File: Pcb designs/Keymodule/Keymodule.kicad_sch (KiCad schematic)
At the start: 105 parts, among them J1 USB connect, U1 RP2040, U2 SN74LV1T34DBV, U3 AMS1117-3.3, U4 W25Q128JVS, Y1 ABM8-272-T3

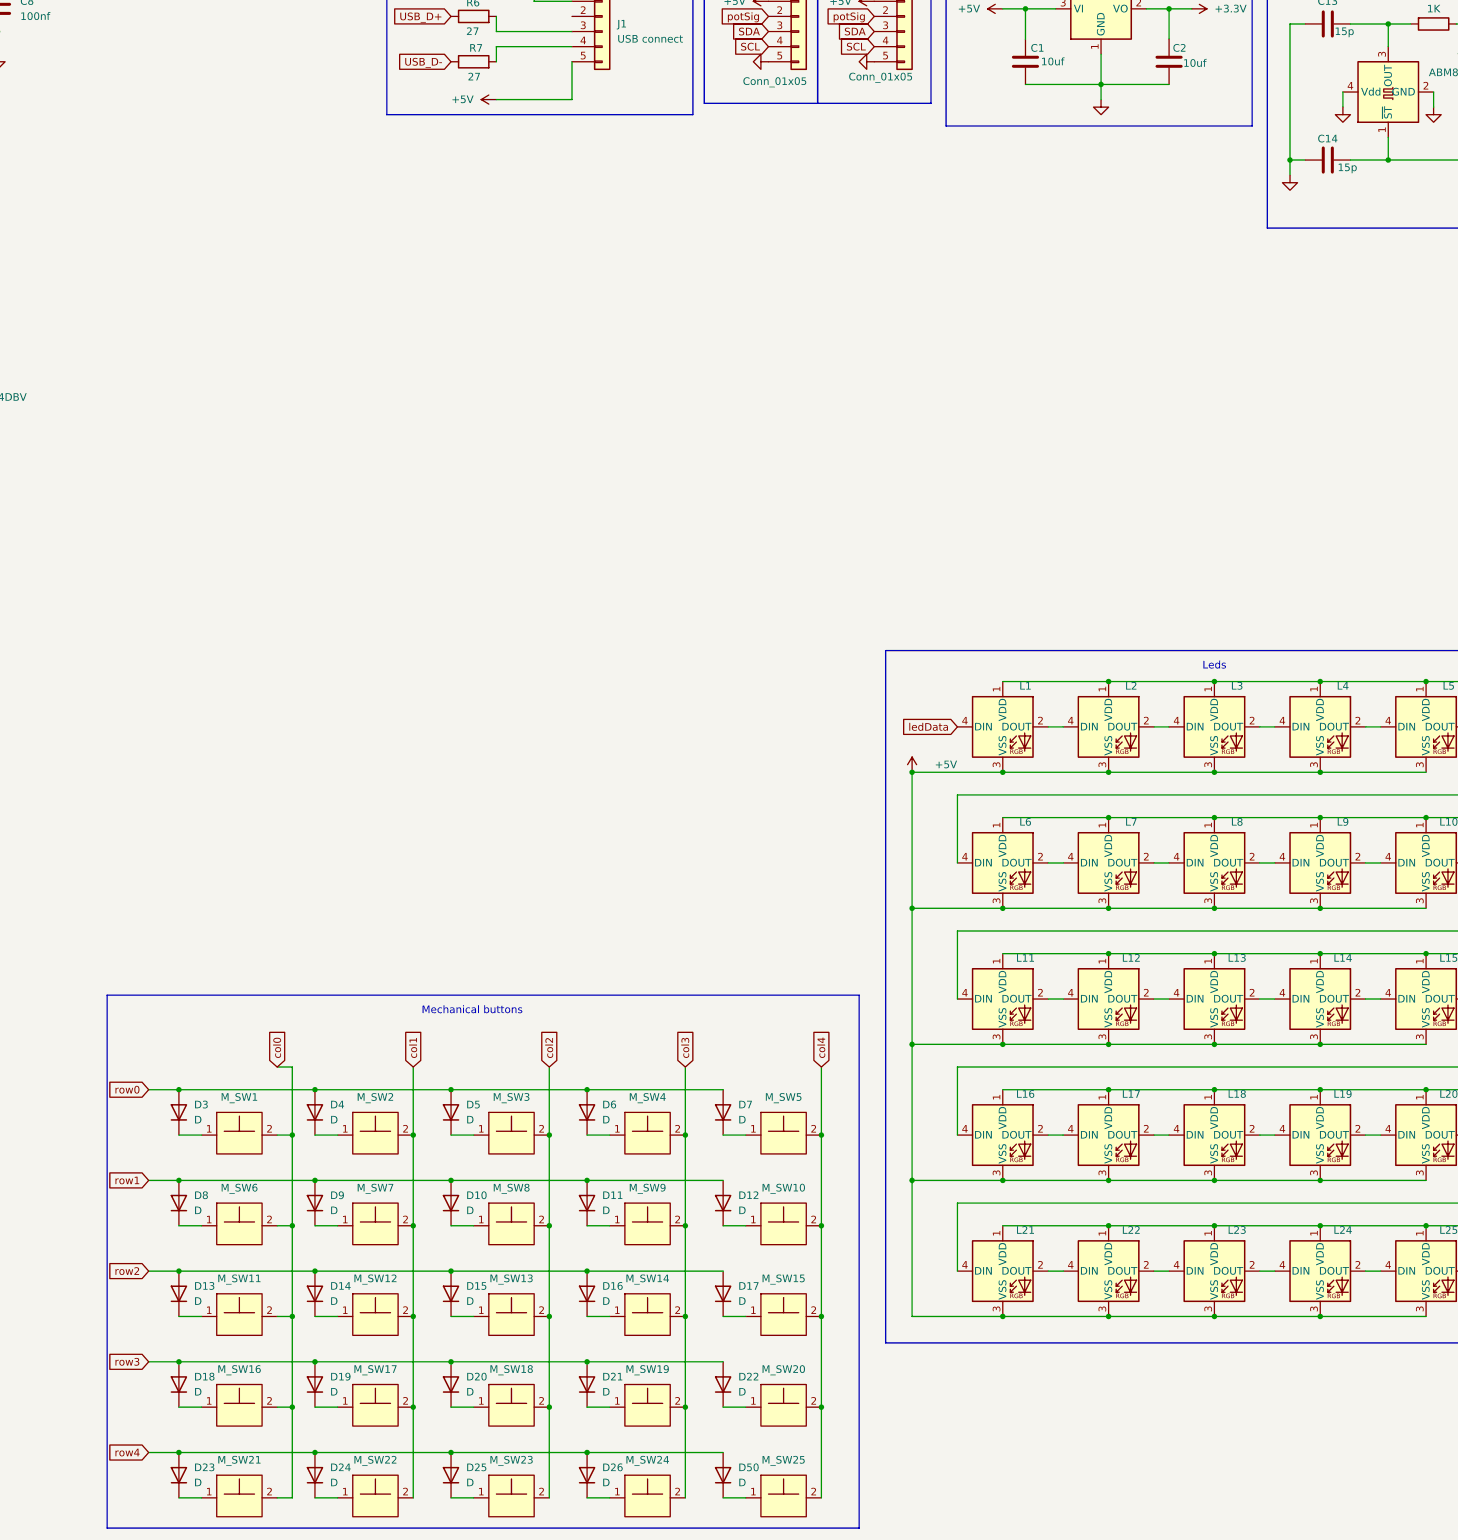
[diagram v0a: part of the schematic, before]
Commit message: Stared wiring ic
LED signal boost not done
But its a start
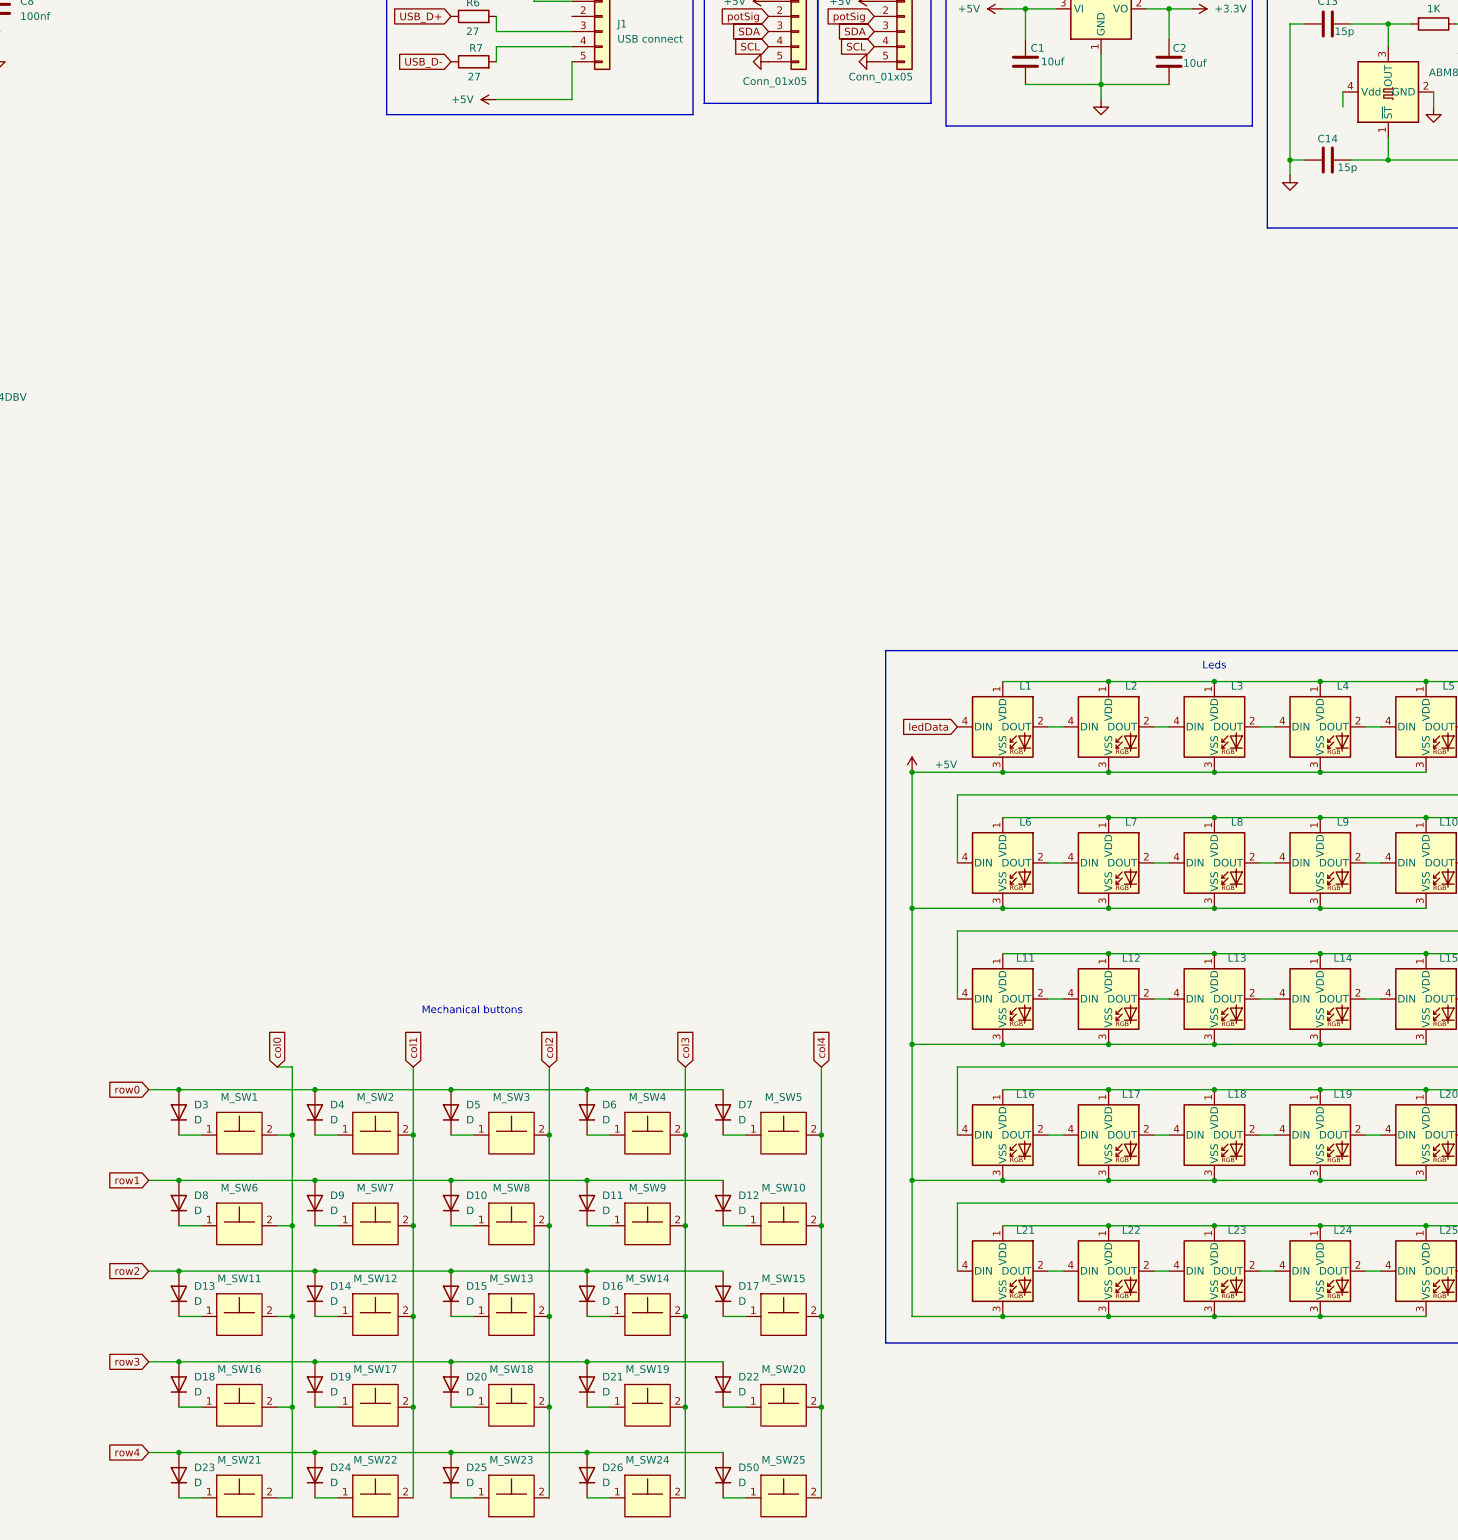
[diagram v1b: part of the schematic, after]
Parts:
- M_SW1, M_SW10, M_SW11, M_SW12, M_SW13, M_SW14, M_SW15, M_SW16, M_SW17, M_SW18, M_SW19, M_SW2, M_SW20, M_SW21, M_SW22, M_SW23, M_SW24, M_SW25, M_SW3, M_SW4, M_SW5, M_SW6, M_SW7, M_SW8, M_SW9: footprint 1_Custom_library:Kailh Switch 1350 -> 1_Custom_library:Kailh low profile Choc switch V1
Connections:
- net GND: no longer Y1.4 (Vdd)
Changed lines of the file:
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@@
 	)
 	(rectangle
-		(start 167.005 191.135)
-		(end 293.37 280.67)
-		(stroke
-			(width 0)
-			(type solid)
-		)
-		(fill
-			(type color)
-			(color 120 120 120 0.38)
-		)
-	)
-	(rectangle
 		(start 213.995 14.605)
 		(end 265.43 43.18)
@@
 			)
 		)
-		(property "Footprint" "1_Custom_library:Kailh Switch 1350"
+		(property "Footprint" "1_Custom_library:Kailh low profile Choc switch V1"
 			(at 280.67 231.14 0)
 			(effects
@@
 			)
 		)
-		(property "Footprint" "1_Custom_library:Kailh Switch 1350"
+		(property "Footprint" "1_Custom_library:Kailh low profile Choc switch V1"
 			(at 212.09 276.86 0)
 			(effects
@@
 			)
 		)
-		(property "Footprint" "1_Custom_library:Kailh Switch 1350"
+		(property "Footprint" "1_Custom_library:Kailh low profile Choc switch V1"
 			(at 234.95 231.14 0)
 			(effects
@@
 			)
 		)
-		(property "Footprint" "1_Custom_library:Kailh Switch 1350"
+		(property "Footprint" "1_Custom_library:Kailh low profile Choc switch V1"
 			(at 189.23 276.86 0)
 			(effects
@@
 			)
 		)
-		(property "Footprint" "1_Custom_library:Kailh Switch 1350"
+		(property "Footprint" "1_Custom_library:Kailh low profile Choc switch V1"
 			(at 234.95 276.86 0)
 			(effects
@@
 			)
 		)
-		(property "Footprint" "1_Custom_library:Kailh Switch 1350"
+		(property "Footprint" "1_Custom_library:Kailh low profile Choc switch V1"
 			(at 212.09 215.9 0)
 			(effects
@@
 			)
 		)
-		(property "Footprint" "1_Custom_library:Kailh Switch 1350"
+		(property "Footprint" "1_Custom_library:Kailh low profile Choc switch V1"
 			(at 189.23 246.38 0)
 			(effects
@@
 			)
 		)
-		(property "Footprint" "1_Custom_library:Kailh Switch 1350"
+		(property "Footprint" "1_Custom_library:Kailh low profile Choc switch V1"
 			(at 257.81 261.62 0)
 			(effects
@@
 			)
 		)
-		(property "Footprint" "1_Custom_library:Kailh Switch 1350"
+		(property "Footprint" "1_Custom_library:Kailh low profile Choc switch V1"
 			(at 257.81 231.14 0)
 			(effects
@@
 			)
 		)
-		(property "Footprint" "1_Custom_library:Kailh Switch 1350"
+		(property "Footprint" "1_Custom_library:Kailh low profile Choc switch V1"
 			(at 280.67 276.86 0)
 			(effects
@@
 			)
 		)
-		(property "Footprint" "1_Custom_library:Kailh Switch 1350"
+		(property "Footprint" "1_Custom_library:Kailh low profile Choc switch V1"
 			(at 257.81 246.38 0)
 			(effects
@@
 			)
 		)
-		(property "Footprint" "1_Custom_library:Kailh Switch 1350"
+		(property "Footprint" "1_Custom_library:Kailh low profile Choc switch V1"
 			(at 257.81 215.9 0)
 			(effects
@@
 			)
 		)
-		(property "Footprint" "1_Custom_library:Kailh Switch 1350"
+		(property "Footprint" "1_Custom_library:Kailh low profile Choc switch V1"
 			(at 189.23 215.9 0)
 			(effects
@@
 			)
 		)
-		(property "Footprint" "1_Custom_library:Kailh Switch 1350"
+		(property "Footprint" "1_Custom_library:Kailh low profile Choc switch V1"
 			(at 189.23 261.62 0)
 			(effects
@@
 			)
 		)
-		(property "Footprint" "1_Custom_library:Kailh Switch 1350"
+		(property "Footprint" "1_Custom_library:Kailh low profile Choc switch V1"
 			(at 212.09 231.14 0)
 			(effects
@@
 			)
 		)
-		(property "Footprint" "1_Custom_library:Kailh Switch 1350"
+		(property "Footprint" "1_Custom_library:Kailh low profile Choc switch V1"
 			(at 257.81 276.86 0)
 			(effects
@@
 			)
 		)
-		(property "Footprint" "1_Custom_library:Kailh Switch 1350"
+		(property "Footprint" "1_Custom_library:Kailh low profile Choc switch V1"
 			(at 234.95 246.38 0)
 			(effects
@@
 			)
 		)
-		(property "Footprint" "1_Custom_library:Kailh Switch 1350"
+		(property "Footprint" "1_Custom_library:Kailh low profile Choc switch V1"
 			(at 234.95 261.62 0)
 			(effects
@@
 	)
 	(symbol
-		(lib_id "power:GND")
-		(at 374.65 41.91 0)
-		(unit 1)
-		(exclude_from_sim no)
-		(in_bom yes)
-		(on_board yes)
-		(dnp no)
-		(fields_autoplaced yes)
-		(property "Reference" "#PWR028"
-			(at 374.65 48.26 0)
-			(effects
-				(font
-					(size 1.27 1.27)
-				)
-				(hide yes)
-			)
-		)
-		(property "Value" "GND"
-			(at 374.65 46.99 0)
-			(effects
-				(font
-					(size 1.27 1.27)
-				)
-				(hide yes)
-			)
-		)
-		(property "Footprint" ""
-			(at 374.65 41.91 0)
-			(effects
-				(font
-					(size 1.27 1.27)
-				)
-				(hide yes)
-			)
-		)
-		(property "Datasheet" ""
-			(at 374.65 41.91 0)
-			(effects
-				(font
-					(size 1.27 1.27)
-				)
-				(hide yes)
-			)
-		)
-		(property "Description" "Power symbol creates a global label with name \"GND\" , ground"
-			(at 374.65 41.91 0)
-			(effects
-				(font
-					(size 1.27 1.27)
-				)
-				(hide yes)
-			)
-		)
-		(pin "1"
-		)
-		(instances
-			(project "Keymodule"
-				(path "/8c3d34a5-d640-4303-a3a8-a4a01dc90234"
-					(reference "#PWR028")
-					(unit 1)
-				)
-			)
-		)
-	)
-	(symbol
 		(lib_id "Device:D")
 		(at 201.93 210.82 90)
@@
 			)
 		)
-		(property "Footprint" "1_Custom_library:Kailh Switch 1350"
+		(property "Footprint" "1_Custom_library:Kailh low profile Choc switch V1"
 			(at 212.09 246.38 0)
 			(effects
@@
 			)
 		)
-		(property "Footprint" "1_Custom_library:Kailh Switch 1350"
+		(property "Footprint" "1_Custom_library:Kailh low profile Choc switch V1"
 			(at 280.67 261.62 0)
 			(effects
@@
 			)
 		)
-		(property "Footprint" "1_Custom_library:Kailh Switch 1350"
+		(property "Footprint" "1_Custom_library:Kailh low profile Choc switch V1"
 			(at 280.67 246.38 0)
 			(effects
@@
 			)
 		)
-		(property "Footprint" "1_Custom_library:Kailh Switch 1350"
+		(property "Footprint" "1_Custom_library:Kailh low profile Choc switch V1"
 			(at 280.67 215.9 0)
 			(effects
@@
 			)
 		)
-		(property "Footprint" "1_Custom_library:Kailh Switch 1350"
+		(property "Footprint" "1_Custom_library:Kailh low profile Choc switch V1"
 			(at 189.23 231.14 0)
 			(effects
@@
 			)
 		)
-		(property "Footprint" "1_Custom_library:Kailh Switch 1350"
+		(property "Footprint" "1_Custom_library:Kailh low profile Choc switch V1"
 			(at 212.09 261.62 0)
 			(effects
@@
 			)
 		)
-		(property "Footprint" "1_Custom_library:Kailh Switch 1350"
+		(property "Footprint" "1_Custom_library:Kailh low profile Choc switch V1"
 			(at 234.95 215.9 0)
 			(effects
